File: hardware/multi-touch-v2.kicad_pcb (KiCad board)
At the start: 2 copper layers, 25 x 30 mm, 31 parts, among them P1 CON-SENSOR2, P2 DEBUG, P3 BOOT, P4 CONN_01X12, U1 MPR121Q, U2 XMC1100, U3 DRILL, U4 DRILL, U5 DRILL, U6 DRILL

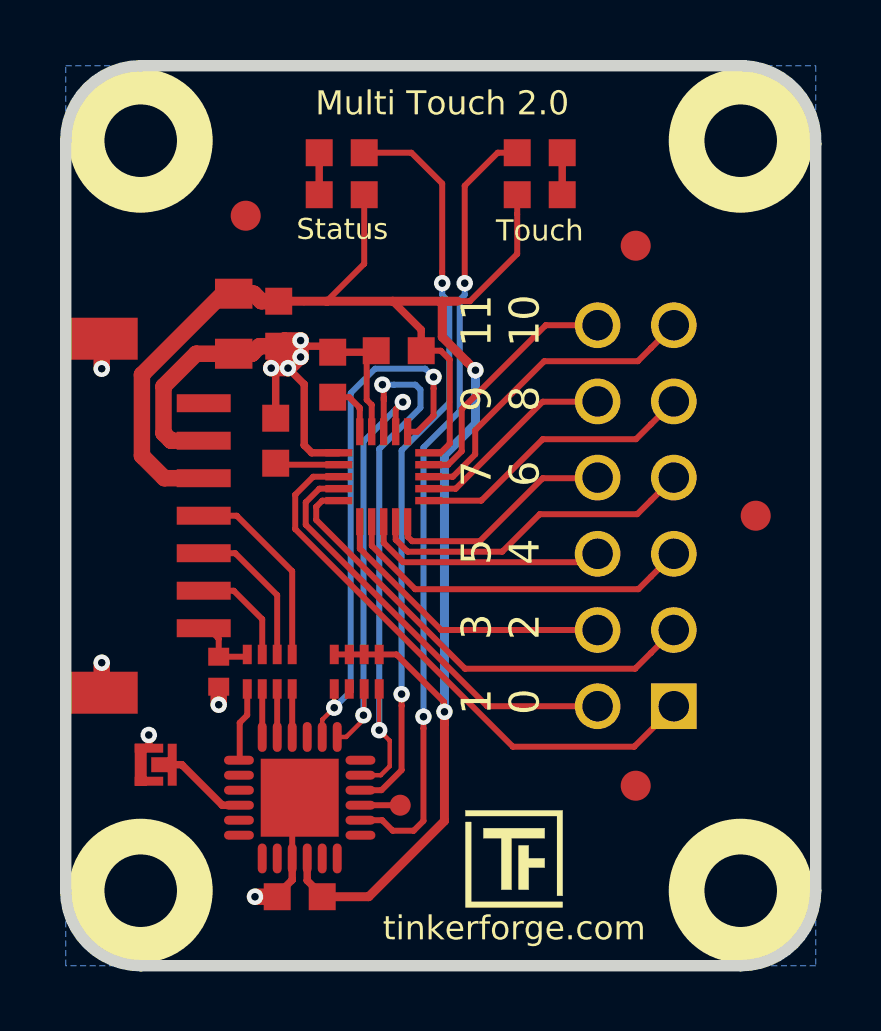
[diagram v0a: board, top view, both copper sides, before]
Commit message: update to new kicad version
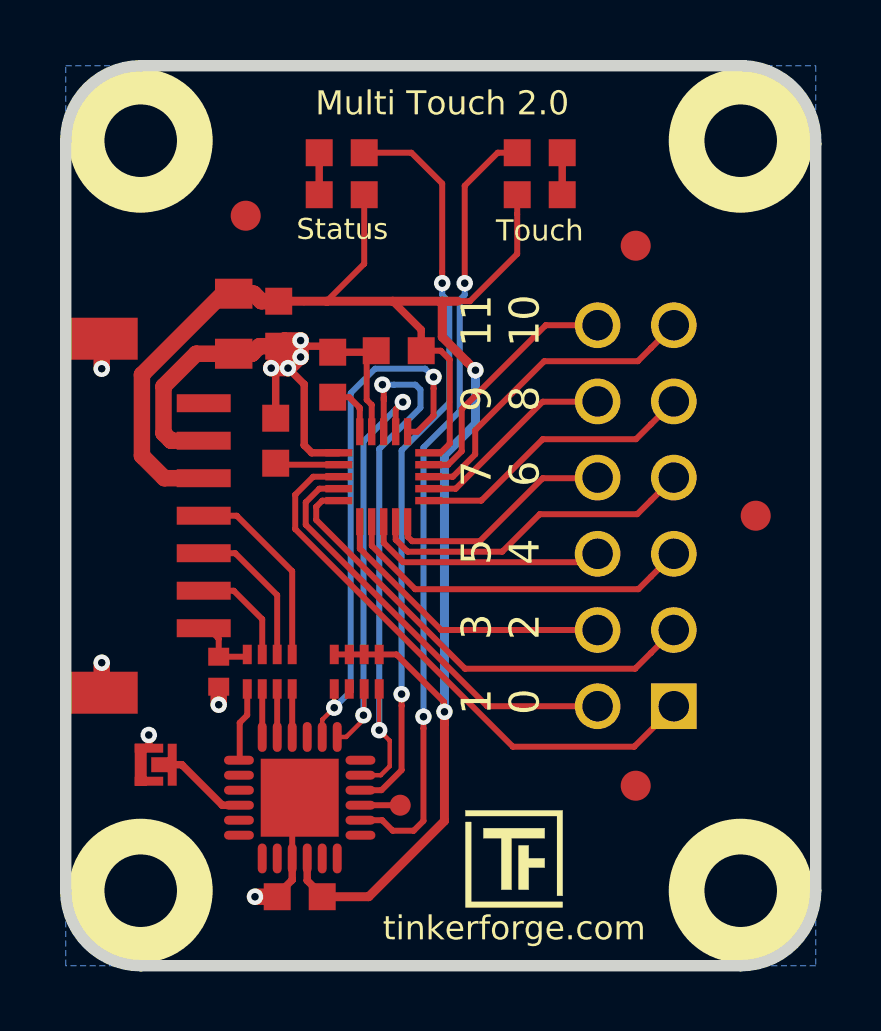
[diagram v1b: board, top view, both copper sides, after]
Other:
- net class Default removed
